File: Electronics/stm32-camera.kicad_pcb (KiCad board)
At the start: 4 copper layers, 36 x 36 mm, 59 parts, among them CON1 MOLEX_47309-2651, P1 HEADER_MALE_2MM_01X06, P2 MOLEX_PICO_PTH_VERT_2_WAY, Q1 VEMT3700, U1 STM32F429VET6, U2 AP2210K-ADJ, U3 AP2210K-ADJ, U4 AP2210K-ADJ, U5 OV02640-VL9A, X1 CSTCE16M0V53A, X2 SWD

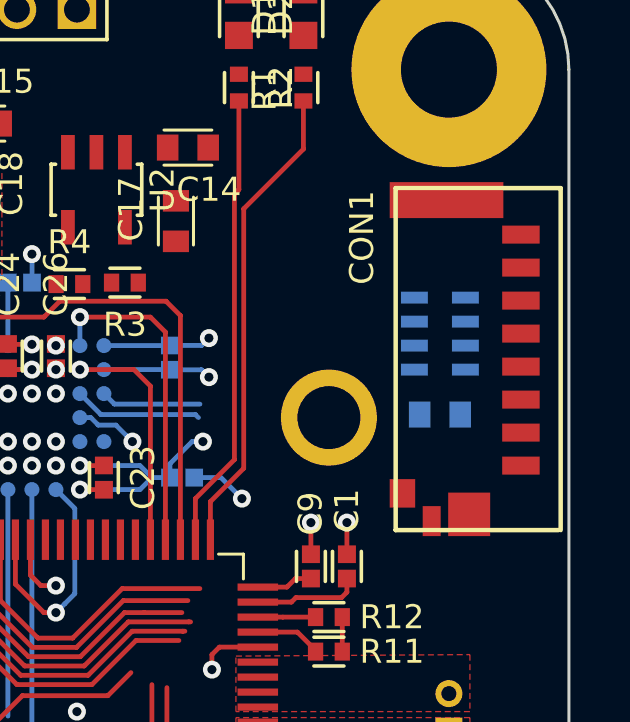
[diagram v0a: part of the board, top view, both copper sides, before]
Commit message: Update loose pcb files
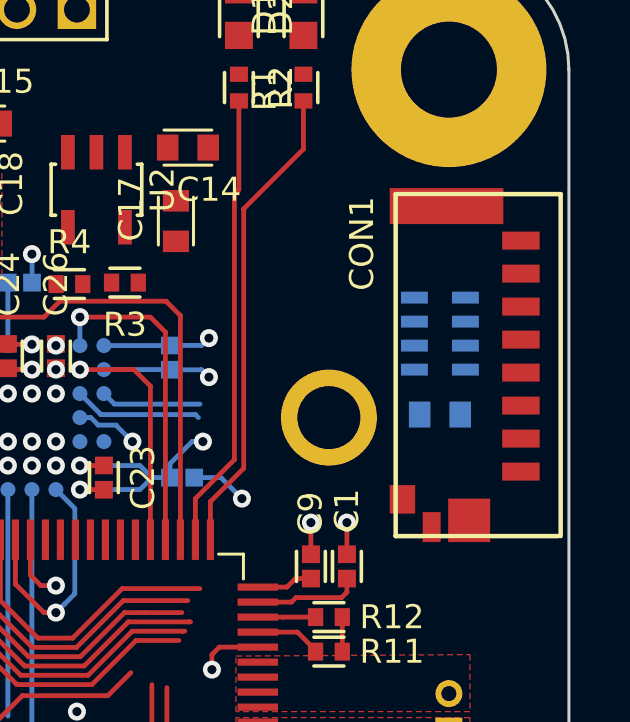
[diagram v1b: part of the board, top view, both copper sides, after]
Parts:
- moved CON1 0.20 mm to (134.4, 113.5)
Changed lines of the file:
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@@
   (general
     (links 185)
-    (no_connects 118)
+    (no_connects 105)
     (area 89.900001 93.54 208.228571 138.767143)
     (thickness 1.6)
@@
     (47 F.CrtYd user hide)
     (48 B.Fab user hide)
-    (49 F.Fab user hide)
+    (49 F.Fab user)
   )
   (setup
@@
   )
   (module Applidyne_Connector_Molex:MOLEX_47309-2651 (layer F.Cu)
-    (at 134.4 113.35 270)
+    (at 134.4 113.55 270)
     (descr http://www.molex.com/pdm_docs/sd/473092651_sd.pdf)
     (tags "SMD SD Card socket compact")
